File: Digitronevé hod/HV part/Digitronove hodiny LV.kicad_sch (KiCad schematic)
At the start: 25 parts, among them J1 StepDown 5V-3,3V, J2 USB C s 5.1k rezitory, J3 Conn_01x05, Q1 MPSA42, Q13 MPSA42, SW1 SW_Push, SW2 SW_Push, SW3 SW_Push, SW4 SW_Push, SW5 SW_Push, U1 74HC595, U2 ESP32-WROOM-32, U3 74HC595, U4 74HC595

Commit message: HV part schematic 01
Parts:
- removed C1: 100 uF, symbol Device:C
- removed C2, C3: 47 uF, symbol Device:C
- removed C4: 4.7 uF, symbol Device:C
- removed F1: Fuse, symbol Device:Fuse
- removed J1: StepDown 5V-3,3V, symbol Connector_Generic:Conn_01x03
- removed J2: USB C s 5.1k rezitory, symbol Connector_Generic:Conn_01x02
- removed J3: Conn_01x05, symbol Connector_Generic:Conn_01x05
- removed Q1, Q13: MPSA42, Package_TO_SOT_THT:TO-92_Inline, symbol Transistor_BJT:MPSA42
- removed R13: 100k, symbol Device:R
- removed R14: 470, symbol Device:R
- removed R4: R_Trim, symbol Device:R_Trim
- removed SW1, SW2, SW3, SW4, SW5: SW_Push, symbol Switch:SW_Push
- removed U2: ESP32-WROOM-32, RF_Module:ESP32-WROOM-32, symbol RF_Module:ESP32-WROOM-32
- removed U3, U4: 74HC595, symbol 74xx:74HC595
- added 170V: Conn_01x02, symbol Connector_Generic:Conn_01x02
- added J1: 3V3, symbol Connector_Generic:Conn_01x01
- added J2: RCLK, symbol Connector_Generic:Conn_01x01
- added J3: SER, symbol Connector_Generic:Conn_01x01
- added J4: SRCLK, symbol Connector_Generic:Conn_01x01
- added J5: 5V, symbol Connector_Generic:Conn_01x01
- added J6, J7: GND, symbol Connector_Generic:Conn_01x01
- added R4: 10K, symbol Device:R
- added U10, U7, U8, U9: IN-14, symbol custom:IN-14
- added U2: 74HC595, symbol 74xx:74HC595
- added U3, U4, U5, U6: ~, symbol custom:K155ID1
- R1: value 470 -> 10K
- R2: value 100k -> 10K
- R3: value 10 k -> 10K
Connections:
- net GND: now also U1.8 (GND), 170V.GND (Pin_2), J6.1 (Pin_1), J7.1 (Pin_1), U2.8 (GND), U3. (Q9), U4. (Q9), U5. (Q9), U6. (Q9); no longer R2.2
- net at R2.1: now also U9. (C_comma); no longer R1.2
- net at R3.1: now also U8. (C_comma)
- net at U1.15 (QA): now also U6. (Q9); no longer R1.1
- net at R3.2: now also R1.2, R2.2, 170V.170V (Pin_1), R4.2
- net at U1.1 (QB): now also U6. (Q9)
- net at U1.11 (SRCLK): now also J4.1 (Pin_1), U2.11 (SRCLK)
- net at U1.12 (RCLK): now also J2.1 (Pin_1), U2.12 (RCLK)
- net at U1.14 (SER): now also J3.1 (Pin_1)
- net at U1.16 (VCC): now also J1.1 (Pin_1), U2.16 (VCC)
- net at U1.2 (QC): now also U6. (Q9)
- net at U1.3 (QD): now also U6. (Q9)
- net at U1.4 (QE): now also U5. (Q9)
- net at U1.5 (QF): now also U5. (Q9)
- net at U1.6 (QG): now also U5. (Q9)
- net at U1.7 (QH): now also U5. (Q9)
- net at U1.9 (QH'): now also U2.14 (SER)
- new net: J5.1 (Pin_1), U3. (Q9), U4. (Q9), U5. (Q9), U6. (Q9)
- new net: U3. (Q9), U7. (C_comma) (x10)
- new net: U2.4 (QE), U3. (Q9)
- new net: U2.5 (QF), U3. (Q9)
- new net: U2.6 (QG), U3. (Q9)
- new net: U2.7 (QH), U3. (Q9)
- new net: R4.1, U7. (C_comma)
- new net: U4. (Q9), U8. (C_comma) (x10)
- new net: U5. (Q9), U9. (C_comma) (x10)
- new net: U2.1 (QB), U4. (Q9)
- new net: U2.15 (QA), U4. (Q9)
- new net: U2.2 (QC), U4. (Q9)
- new net: U2.3 (QD), U4. (Q9)
- new net: R1.1, U10. (C_comma)
- new net: U10. (C_comma), U6. (Q9) (x10)
- no-connect marks 3 -> 10

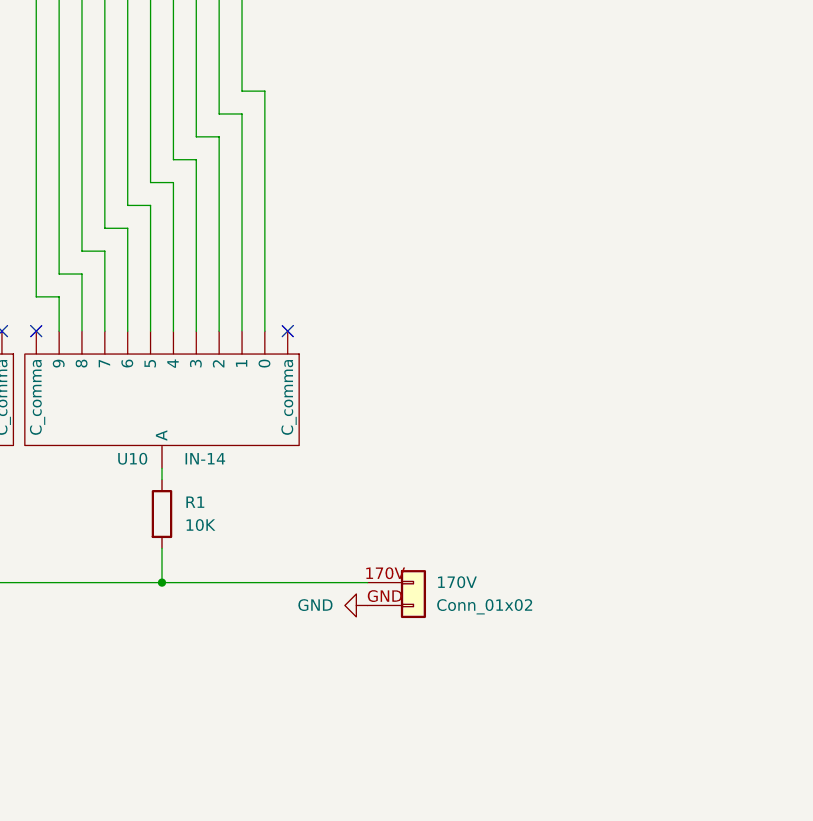
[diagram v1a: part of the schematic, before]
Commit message: HV scheme update
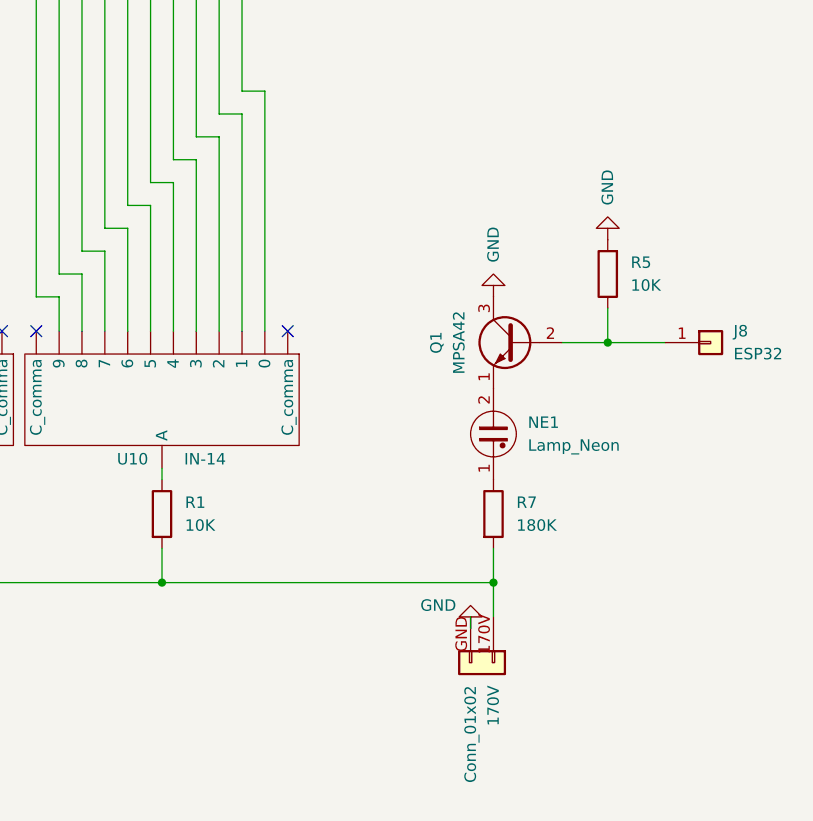
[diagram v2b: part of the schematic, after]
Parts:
- added J8: ESP32, symbol Connector_Generic:Conn_01x01
- added NE1: Lamp_Neon, symbol Device:Lamp_Neon
- added Q1: MPSA42, Package_TO_SOT_THT:TO-92_Inline, symbol Transistor_BJT:MPSA42
- added R5: 10K, symbol Device:R
- added R7: 180K, symbol Device:R
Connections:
- net GND: now also Q1.3 (C), R5.2
- net at U7. (C_comma): now also R4.1; no longer U3. (Q9)
- net at U8. (C_comma): now also R3.1
- net at U9. (C_comma): now also R2.1
- net at 170V.170V (Pin_1), R1.2, R2.2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: now also R7.2
- net at U10. (C_comma): no longer U6. (Q9)
- new net: J8.1 (Pin_1), Q1.2 (B), R5.1
- new net: J5.1 (Pin_1), U3. (Q9), U4. (Q9), U5. (Q9), U6. (Q9)
- new net: U3. (Q9), U7. (C_comma) (x10)
- new net: U4. (Q9), U8. (C_comma) (x10)
- new net: NE1.1, R7.1
- new net: NE1.2, Q1.1 (E)
- new net: U5. (Q9), U9. (C_comma) (x10)
- new net: U10. (C_comma), U6. (Q9) (x10)
- now unconnected: U10. (C_comma), U10. (C_comma), U10. (C_comma), U10. (C_comma), U10. (C_comma), U10. (C_comma), U10. (C_comma), U10. (C_comma), U10. (C_comma)
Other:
- moved on the sheet: 170V

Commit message: LV update
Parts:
- U1, U2: footprint (none) -> LOGIC-74HC595N_DIP16_:74HC595N
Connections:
- net at U7. (C_comma): now also R4.1; no longer U3. (Q9)
- net at U8. (C_comma): now also R3.1
- net at U9. (C_comma): now also R2.1
- net at U10. (C_comma): no longer U6. (Q9)
- new net: J5.1 (Pin_1), U3. (Q9), U4. (Q9), U5. (Q9), U6. (Q9)
- new net: U3. (Q9), U7. (C_comma) (x10)
- new net: U4. (Q9), U8. (C_comma) (x10)
- new net: U5. (Q9), U9. (C_comma) (x10)
- new net: U10. (C_comma), U6. (Q9) (x10)
- now unconnected: U10. (C_comma), U10. (C_comma), U10. (C_comma), U10. (C_comma), U10. (C_comma), U10. (C_comma), U10. (C_comma), U10. (C_comma), U10. (C_comma)
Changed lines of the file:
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@@
 			)
 		)
-		(property "Footprint" ""
+		(property "Footprint" "LOGIC-74HC595N_DIP16_:74HC595N"
 			(at 110.49 49.53 0)
 			(effects
@@
 			)
 		)
-		(property "Footprint" ""
+		(property "Footprint" "LOGIC-74HC595N_DIP16_:74HC595N"
 			(at 58.42 49.53 0)
 			(effects
